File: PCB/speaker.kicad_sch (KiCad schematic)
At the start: 2 parts, among them U2 MAX98357A

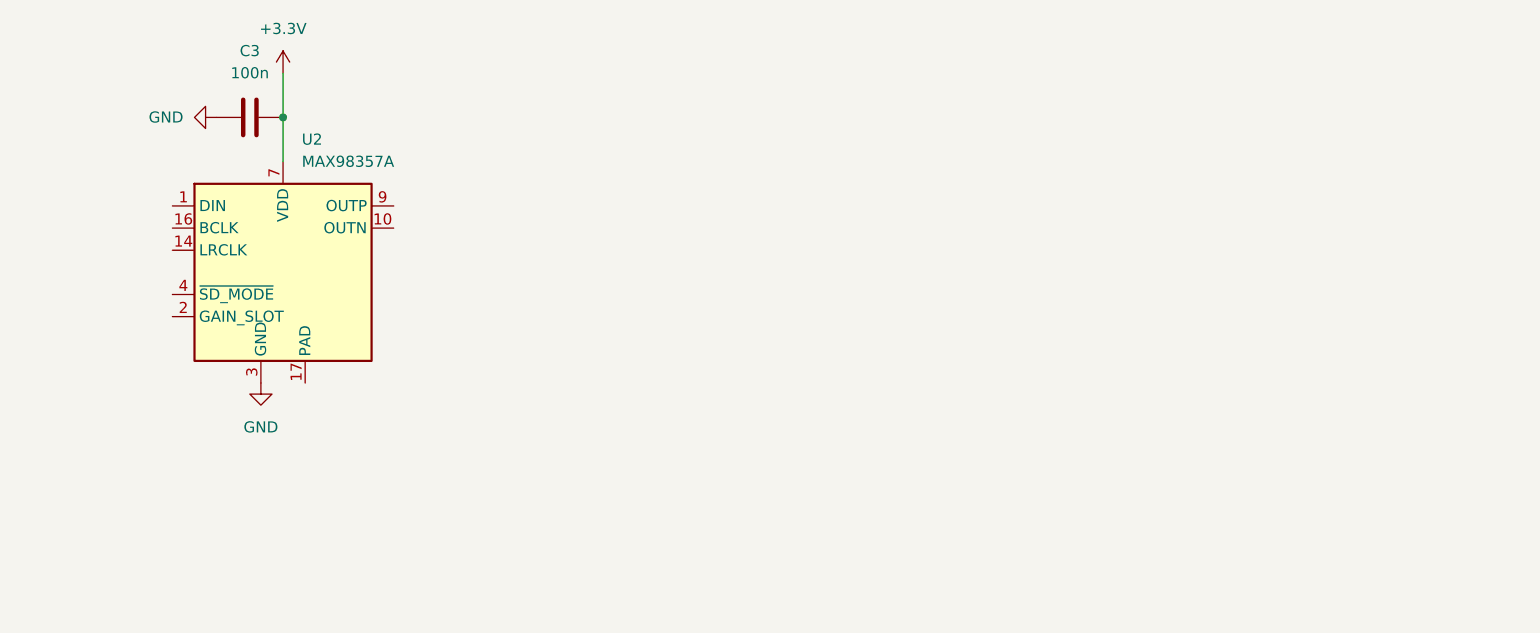
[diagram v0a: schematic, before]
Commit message: schematic
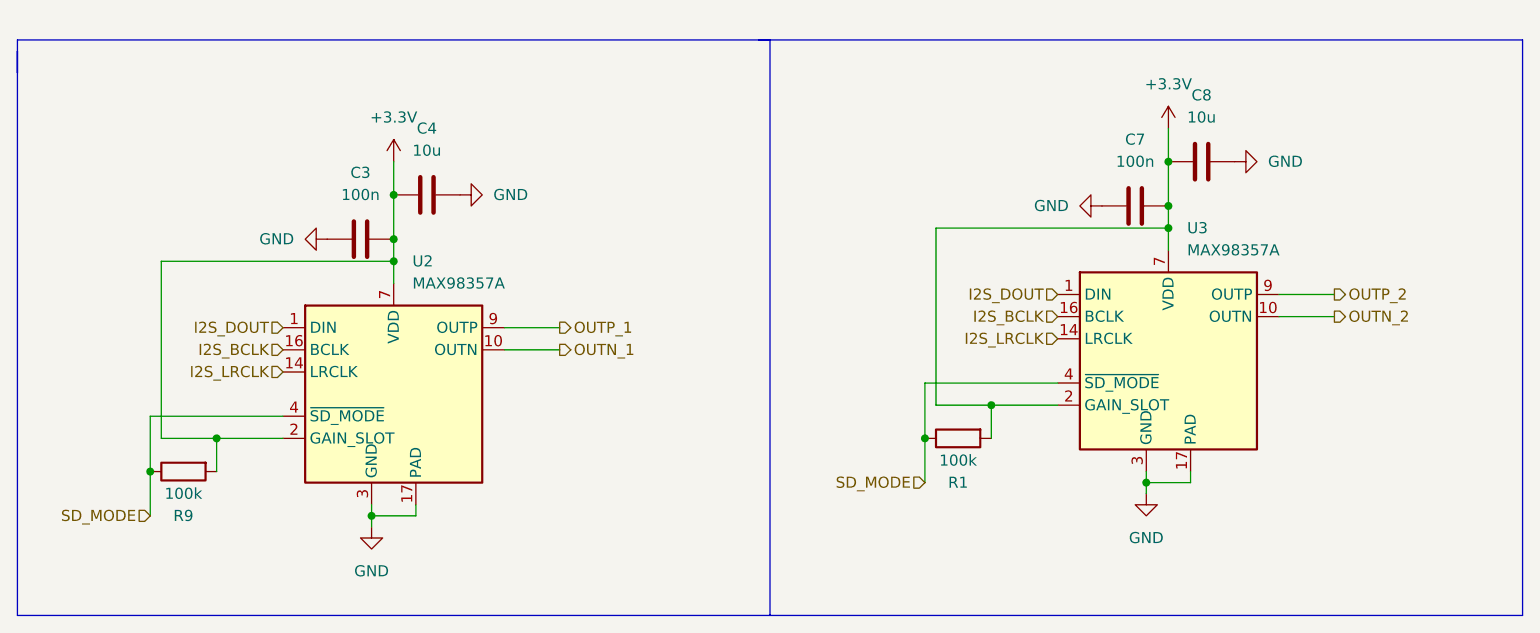
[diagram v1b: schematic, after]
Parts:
- added C4, C8: 10u, Capacitor_SMD:C_0805_2012Metric, symbol Device:C
- added C7: 100n, Capacitor_SMD:C_0603_1608Metric_Pad1.08x0.95mm_HandSolder, symbol Device:C
- added R1, R9: 100k, Resistor_SMD:R_0603_1608Metric, symbol Device:R
- added U3: MAX98357A, Package_DFN_QFN:TQFN-16-1EP_3x3mm_P0.5mm_EP1.23x1.23mm, symbol Audio:MAX98357A
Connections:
- net +3.3V: now also U2.2 (GAIN_SLOT), C4.2, C7.2, C8.2, R1.2, R9.2, U3.2 (GAIN_SLOT), U3.7 (VDD), U3.8 (VDD)
- net GND: now also U2.17 (PAD), C4.1, C7.1, C8.1, U3.11 (GND), U3.15 (GND), U3.17 (PAD), U3.3 (GND)
- net I2S_DOUT: now reaches U2.1 (DIN)
- net I2S_DOUT: now also U3.1 (DIN)
- net OUTN_1: now reaches U2.10 (OUTN)
- net I2S_LRCLK: now reaches U2.14 (LRCLK)
- net I2S_LRCLK: now also U3.14 (LRCLK)
- net I2S_BCLK: now reaches U2.16 (BCLK)
- net I2S_BCLK: now also U3.16 (BCLK)
- net SD_MODE: now reaches U2.4 (~{SD_MODE})
- net SD_MODE: now also R1.1, R9.1, U3.4 (~{SD_MODE})
- net OUTP_1: now reaches U2.9 (OUTP)
- new net OUTN_2: U3.10 (OUTN)
- new net OUTP_2: U3.9 (OUTP)
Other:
- moved on the sheet: C3, U2
